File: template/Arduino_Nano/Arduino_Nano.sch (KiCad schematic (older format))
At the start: 6 parts, among them P1 Digital, P2 Analog, P3 CONN_1, P4 CONN_1, P5 CONN_1, P6 CONN_1

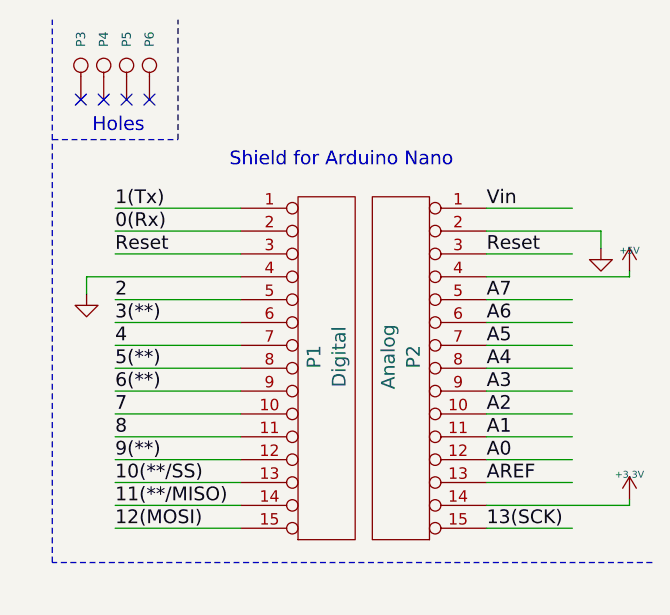
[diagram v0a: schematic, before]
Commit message: Correction schématics
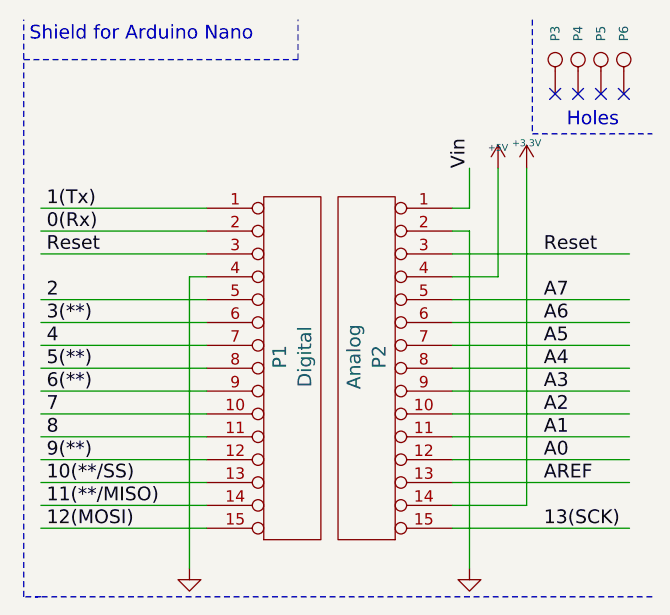
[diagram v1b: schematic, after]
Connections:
- wire segments 34 -> 35
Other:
- moved on the sheet: P1, P2, P3, P4, P5, P6

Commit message: rebuilt shematic and fix librairie
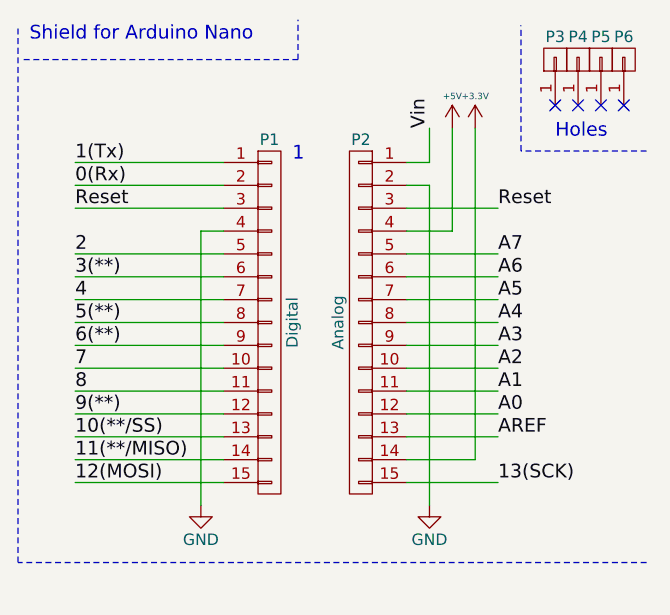
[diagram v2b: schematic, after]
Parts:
- removed P1: Digital, Socket_Arduino_Nano:Socket_Strip_Arduino_1x15, symbol CONN_15
- removed P2: Analog, Socket_Arduino_Nano:Socket_Strip_Arduino_1x15, symbol CONN_15
- removed P3, P4, P5, P6: CONN_1, Socket_Arduino_Nano:1pin_Nano, symbol CONN_1
- added P1: Digital, Socket_Arduino_Nano:Socket_Strip_Arduino_1x15, symbol CONN_01X15
- added P2: Analog, Socket_Arduino_Nano:Socket_Strip_Arduino_1x15, symbol CONN_01X15
- added P3, P4, P5, P6: CONN_01X01, Socket_Arduino_Nano:1pin_Nano, symbol CONN_01X01
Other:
- note added: "1"
